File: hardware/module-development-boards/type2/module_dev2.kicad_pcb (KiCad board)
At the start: 2 copper layers, 30 x 26 mm, 32 parts, among them J1 SensorHub_Module_CONN_V1, J12 Conn_01x01, J13 Conn_01x01, J14 Conn_01x01, J15 Conn_01x01, J16 Conn_01x01, J17 Conn_01x01, J18 Conn_01x01, J19 Conn_01x01, J2 Conn_01x08, J21 Conn_01x01, J22 Conn_01x01, J24 Conn_01x01, J25 Conn_01x01, J26 Conn_01x01, J27 Conn_01x01, J28 Conn_01x01, J29 Conn_01x01, J3 Conn_01x08, J30 Conn_01x01, J31 Conn_01x01, J32 Conn_01x01, J4 Conn_01x08, J5 Conn_01x08, J6 Conn_01x08, J7 Conn_01x05, J8 Conn_01x05

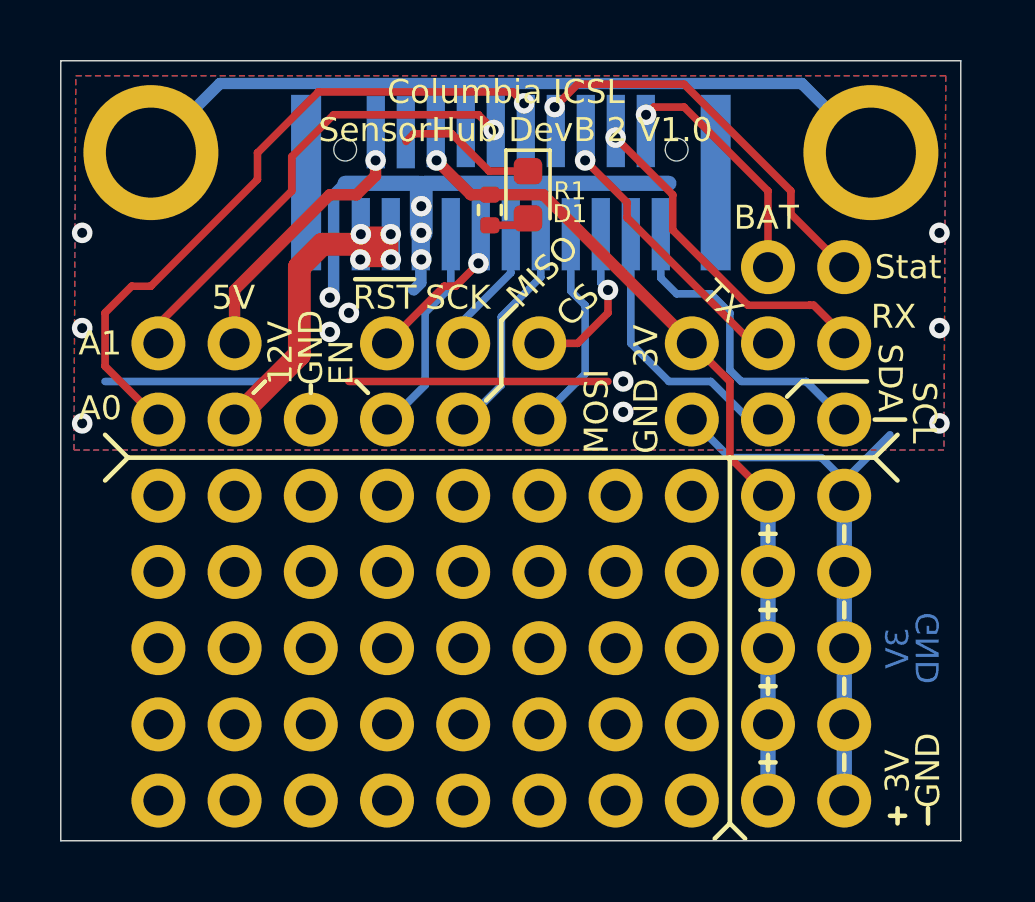
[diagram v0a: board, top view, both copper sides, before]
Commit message: cleanup dev board type 2
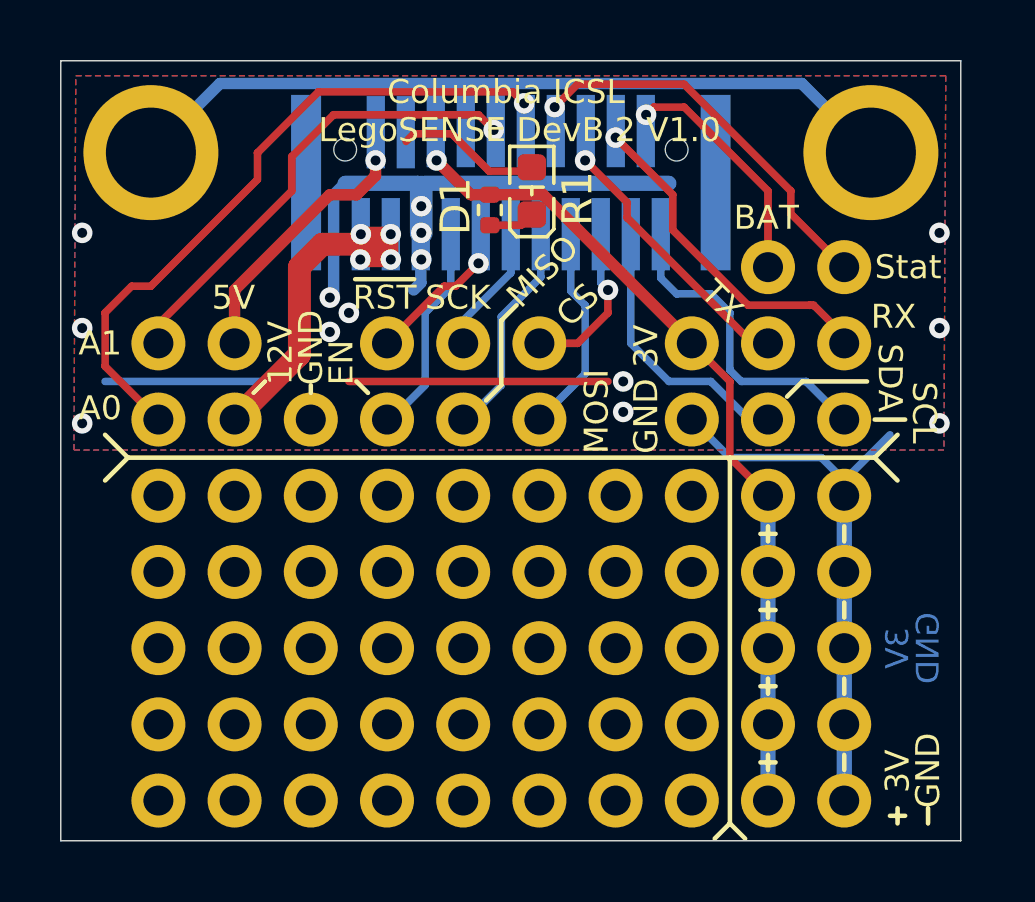
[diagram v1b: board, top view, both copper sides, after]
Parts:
- D1: value D_LED_0603_Red -> LED_0603_Red; footprint LED_SMD:LED_0603_1608Metric -> jlcsmt:LED_0603_1608Metric
- J1: value SensorHub_Module_CONN_V1 -> LegoSENSE_Module_CONN_V1
- moved D1 0.18 mm to (107.7, 65.3), turned to 90 degrees
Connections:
- net /~RST renamed /~{RST}
- D1 pad 2: Net-(D1-Pad2) -> (no net)
- R1 pad 2: Net-(D1-Pad2) -> (no net)
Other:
- net class Default removed
- board text added: "LegoSENSE DevB 2 V1.0"
- board text added: "~{RST}"
- board text removed: "SensorHub DevB 2 V1.0"
- board text removed: "~RST"
